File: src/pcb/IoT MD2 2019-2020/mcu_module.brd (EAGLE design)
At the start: 44.4 x 60.6 mm, 21 parts, among them IC2 ATSAMD21G18A-AU, Y1 ABS07-32.768KHZ-T

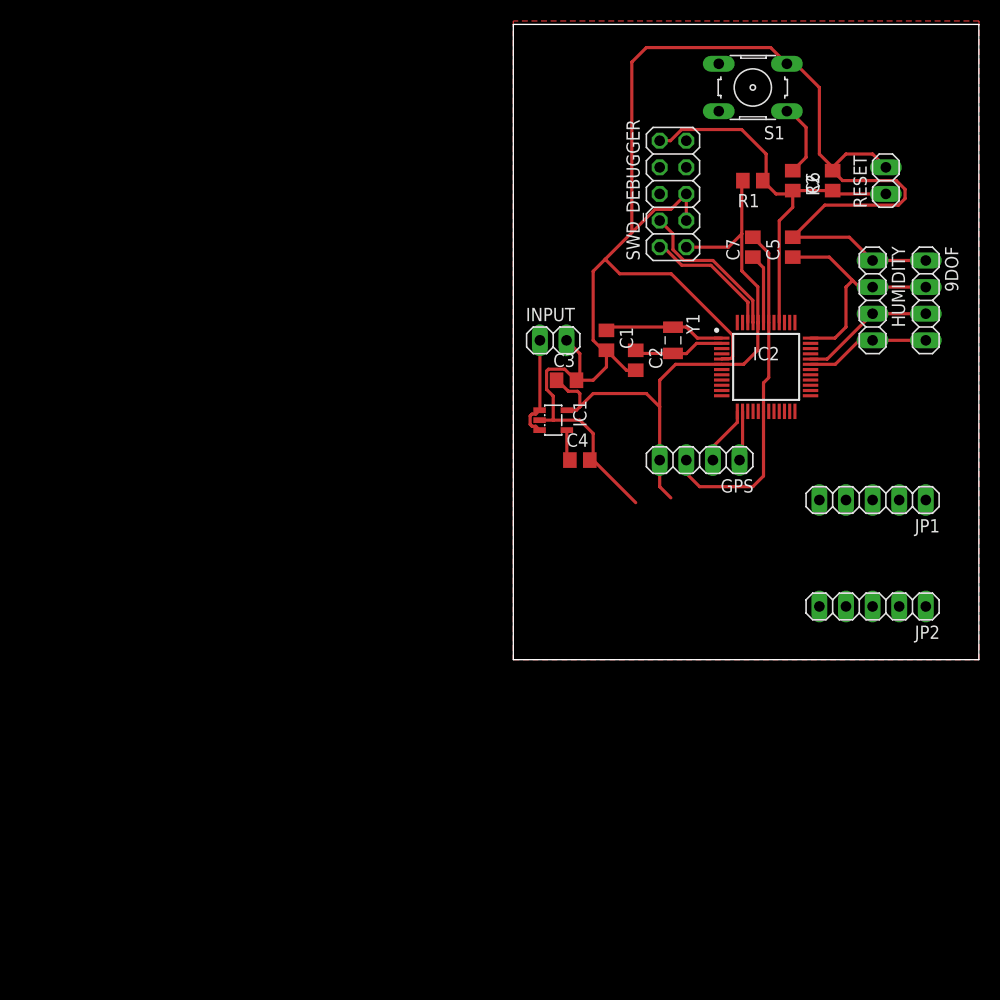
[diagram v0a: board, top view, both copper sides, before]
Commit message: MCU PCB v3
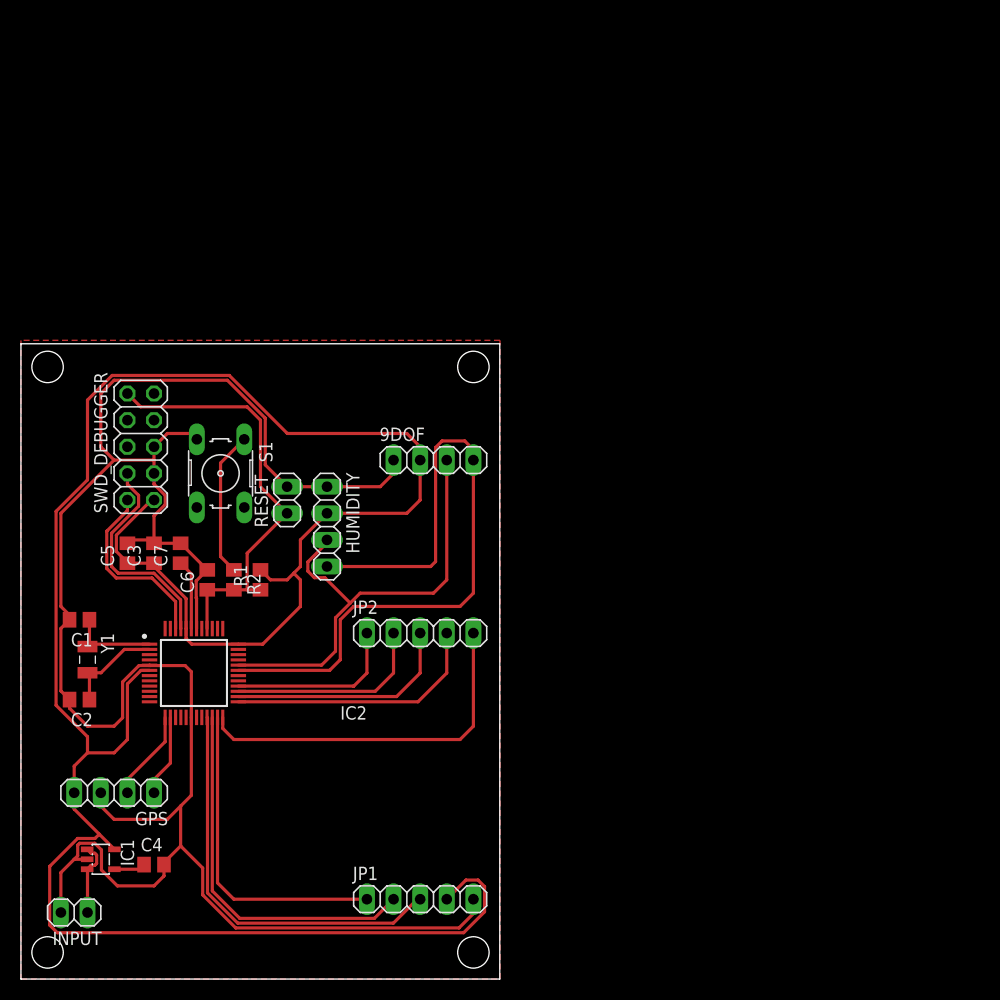
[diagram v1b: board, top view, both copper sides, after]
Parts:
- moved INPUT 71.2 mm to (15.2, 1.27), turned to 180 degrees
- moved C6 70.8 mm to (27.9, 33.0)
- moved C5 69.9 mm to (20.3, 35.6)
- moved R2 65.5 mm to (30.5, 33.0)
- moved RESET 64.8 mm to (35.6, 40.6)
- moved GPS 64.3 mm to (19.1, 12.7)
- moved Y1 63.7 mm to (16.5, 25.4)
- moved S1 62.7 mm to (29.2, 43.2), turned to 270 degrees
- moved C2 62.2 mm to (15.7, 21.6), turned to 180 degrees
- moved C7 61.9 mm to (25.4, 35.6)
- moved IC2 61.9 mm to (26.7, 24.1)
- moved R1 60.5 mm to (33.0, 33.0), turned to 90 degrees
- moved IC1 60.2 mm to (17.8, 6.35)
- moved JP1 57.6 mm to (48.3, 2.54), turned to 0 degrees
- moved C1 56.9 mm to (15.7, 29.2), turned to 180 degrees
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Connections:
- net DIO0: now also JP1.3; no longer JP1.5
- net DIO1: now also JP1.2; no longer JP1.4
- net DIO2: now also JP1.1; no longer JP1.3
- net GND: now also JP1.5; no longer JP2.4
- net MISO: now also JP2.1; no longer JP2.3
- net MOSI: now also IC2.27, JP2.2; no longer IC2.25, JP1.1
- net NSS: now also IC2.25, JP2.4; no longer IC2.27, JP2.2
- net RESET_LORA: now also JP2.5; no longer JP1.2
- net SCK: now also JP2.3; no longer JP2.1
- net SCL: now also 9DOF.4, HUMIDITY.4, IC2.31; no longer 9DOF.3, HUMIDITY.3, IC2.32
- net SDA: now also 9DOF.3, HUMIDITY.3, IC2.32; no longer 9DOF.4, HUMIDITY.4, IC2.31
- net VDD: now also JP1.4; no longer JP2.5
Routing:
- net VDD: track 81.2 -> 217.1 mm
- net SCL: track 12.8 -> 67.1 mm
- net DIO0: track 0.00 -> 39.2 mm
- net DIO1: track 0.00 -> 35.7 mm
- net RESET_LORA: track 0.00 -> 34.8 mm
- net SDA: track 12.0 -> 45.6 mm
- net DIO2: track 0.00 -> 30.7 mm
- net NSS: track 0.00 -> 24.8 mm
- net SCK: track 0.00 -> 22.1 mm
- net MOSI: track 0.00 -> 19.3 mm
- net MISO: track 0.00 -> 16.6 mm
- net GND: track 195.7 -> 206.5 mm
- net N$3: track 7.13 -> 13.9 mm
- net SWDCLK: track 15.1 -> 21.1 mm
- net SWDIO: track 12.6 -> 17.8 mm
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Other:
- board size 44.4 x 60.6 mm -> 45.7 x 60.6 mm
